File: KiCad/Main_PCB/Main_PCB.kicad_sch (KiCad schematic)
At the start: 18 parts, among them J2 USB_C_Receptacle_USB2.0_14P, Q1 S8050, Q2 S8050, U1 ESP32-PICO-D4, U2 CP2102N-Axx-xQFN28

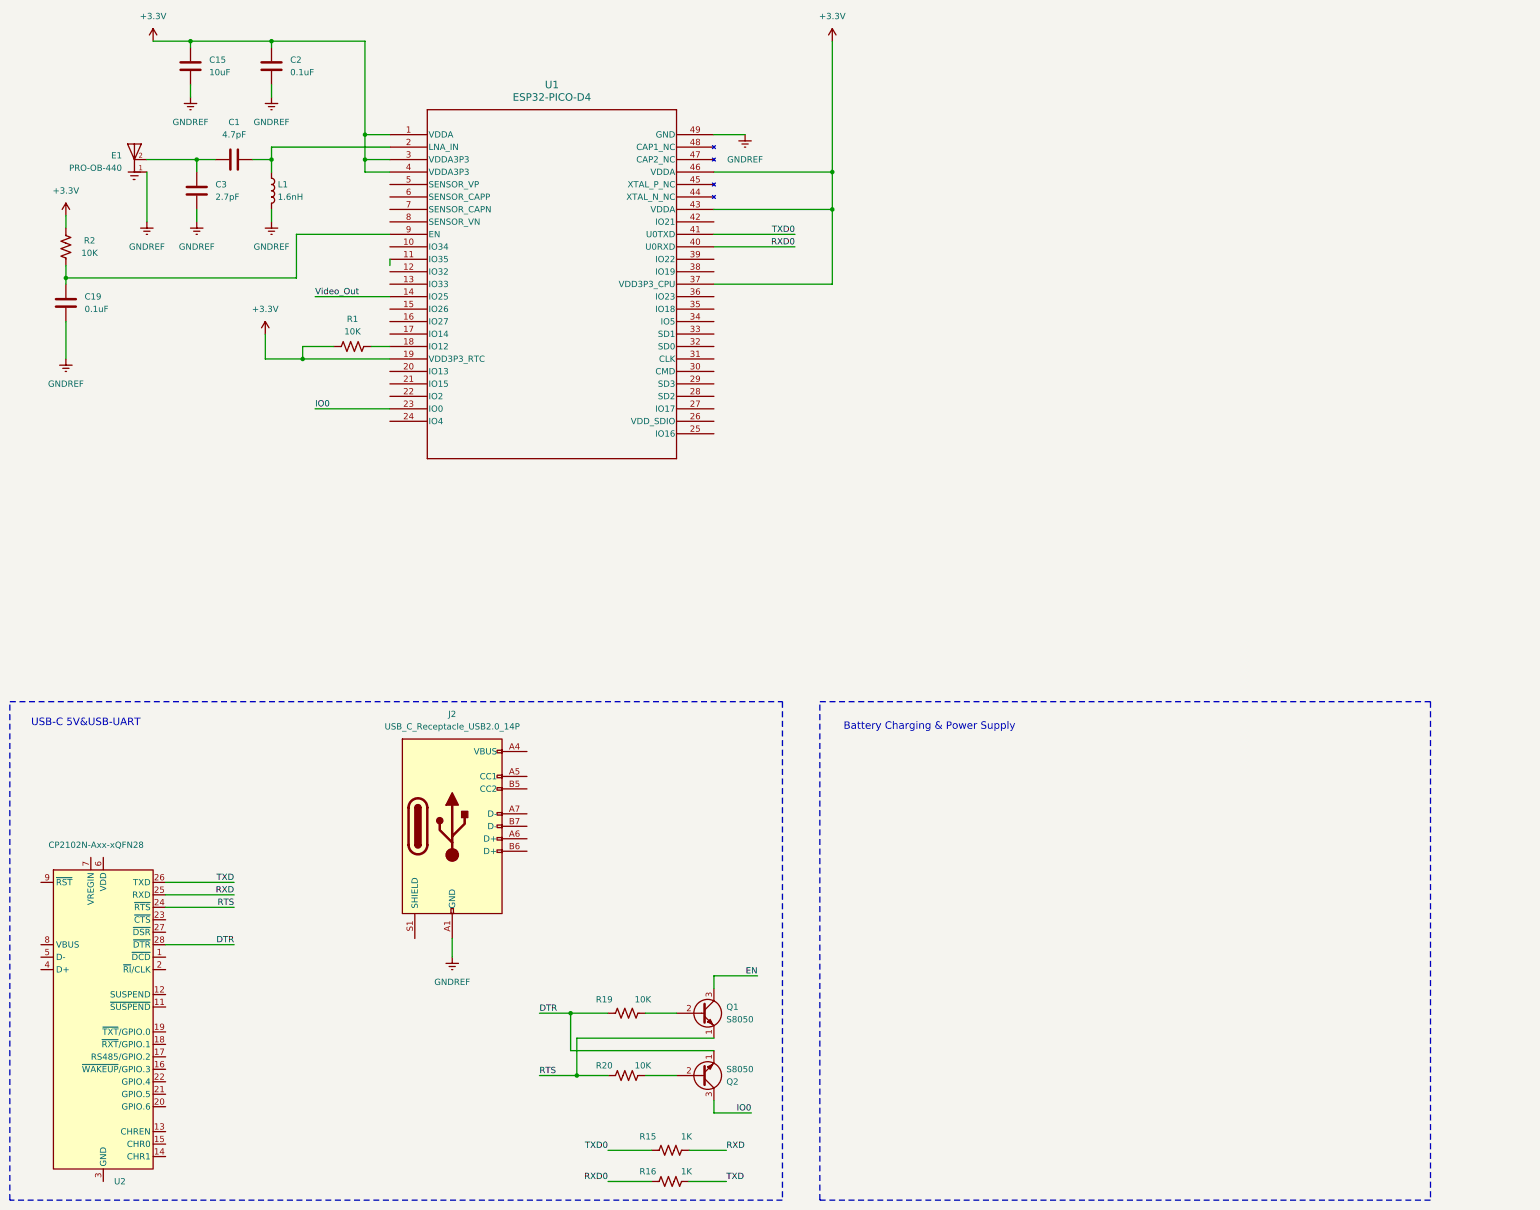
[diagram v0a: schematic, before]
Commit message: Updated PCB
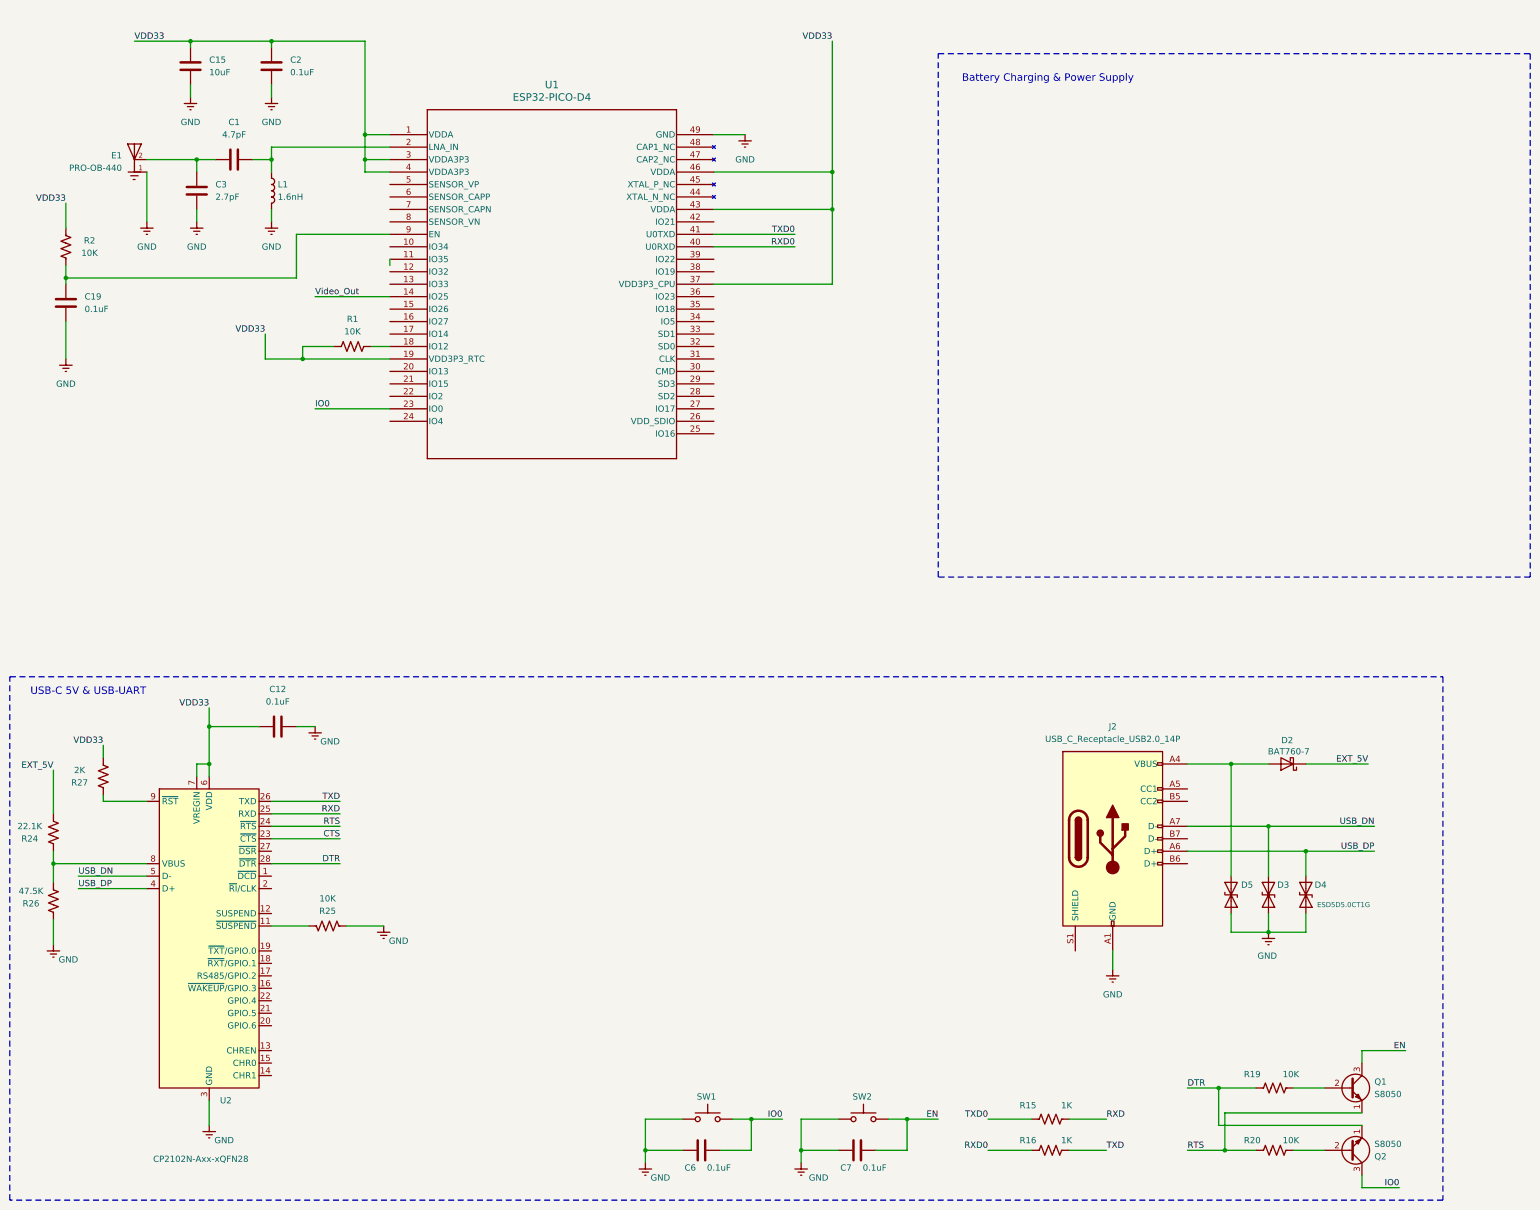
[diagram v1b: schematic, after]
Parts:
- added C12, C6, C7: 0.1uF, symbol Device:C
- added D2: BAT760-7, symbol Device:D_Schottky
- added D3, D4, D5: ESD5D5.0CT1G, Diode_SMD:D_SOD-923, symbol Diode:ESD9B3.3ST5G
- added R24: 22.1K, symbol Device:R_US
- added R25: 10K, symbol Device:R_US
- added R26: 47.5K, symbol Device:R_US
- added R27: 2K, symbol Device:R_US
- added SW1, SW2: ~, symbol Switch:SW_Push
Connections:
- net +3.3V is gone; now on net VDD33: C15.1, C2.1, R1.1, R2.1, U1.1 (VDDA), U1.19 (VDD3P3_RTC), U1.3 (VDDA3P3), U1.37 (VDD3P3_CPU), U1.4 (VDDA3P3), U1.43 (VDDA), U1.46 (VDDA)
- net GNDREF is gone; now on net GND: C15.2, C19.2, C2.2, C3.2, E1.1, J2.A1 (GND), J2.A12 (GND), J2.B1 (GND), J2.B12 (GND), L1.2, U1.49 (GND)
- net EN: now also C7.1, SW2.2
- net IO0: now also C6.1, SW1.2
- net at U2.11 (~{SUSPEND}): now also R25.1
- net CTS: now reaches U2.23 (~{CTS})
- net GND: now reaches U2.29 (GND), U2.3 (GND)
- net GND: now also C12.2, C6.2, C7.2, D3.2 (A2), D4.2 (A2), D5.2 (A2), R25.2, R26.2, SW1.1, SW2.1
- net USB_DP: now reaches U2.4 (D+)
- net USB_DP: now also J2.A6 (D+), D4.1 (A1)
- net USB_DN: now reaches U2.5 (D-)
- net USB_DN: now also J2.A7 (D-), D3.1 (A1)
- net VDD33: now reaches U2.6 (VDD)
- net VDD33: now also U2.7 (VREGIN), C12.1, R27.1
- net at U2.8 (VBUS): now also R24.2, R26.1
- net at U2.9 (~{RST}): now also R27.2
- net at J2.A4 (VBUS), J2.A9 (VBUS), J2.B4 (VBUS)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: now also D2.2 (A), D5.1 (A1)
- new net EXT_5V: D2.1 (K), R24.1
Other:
- note added: "USB-C 5V & USB-UART"
- note removed: "USB-C 5V&USB-UART"
- moved on the sheet: J2, Q1, Q2, R15, R16, R19, R20, U2
